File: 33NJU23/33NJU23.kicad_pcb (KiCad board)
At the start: 2 copper layers, 54 x 85.7 mm, 75 parts, among them CN1 HDMI, J1 VGA, J10 Conn_01x02, J11 Conn_01x01, J12 Audio OUT, J13 Audio IN, J14 JOY-1, J15 USB_A, J17 USB_B_Micro, J18 Conn_01x02_Female, J2 EXT, J3 Micro_SD_Card, J4 Conn_SD, J5 PWR, J6 UART, J7 Mini-DIN-6, J8 IN_A, J9 IN_A, Q1 BC850, Q2 BC850, U1 raspberrypi-pico-module

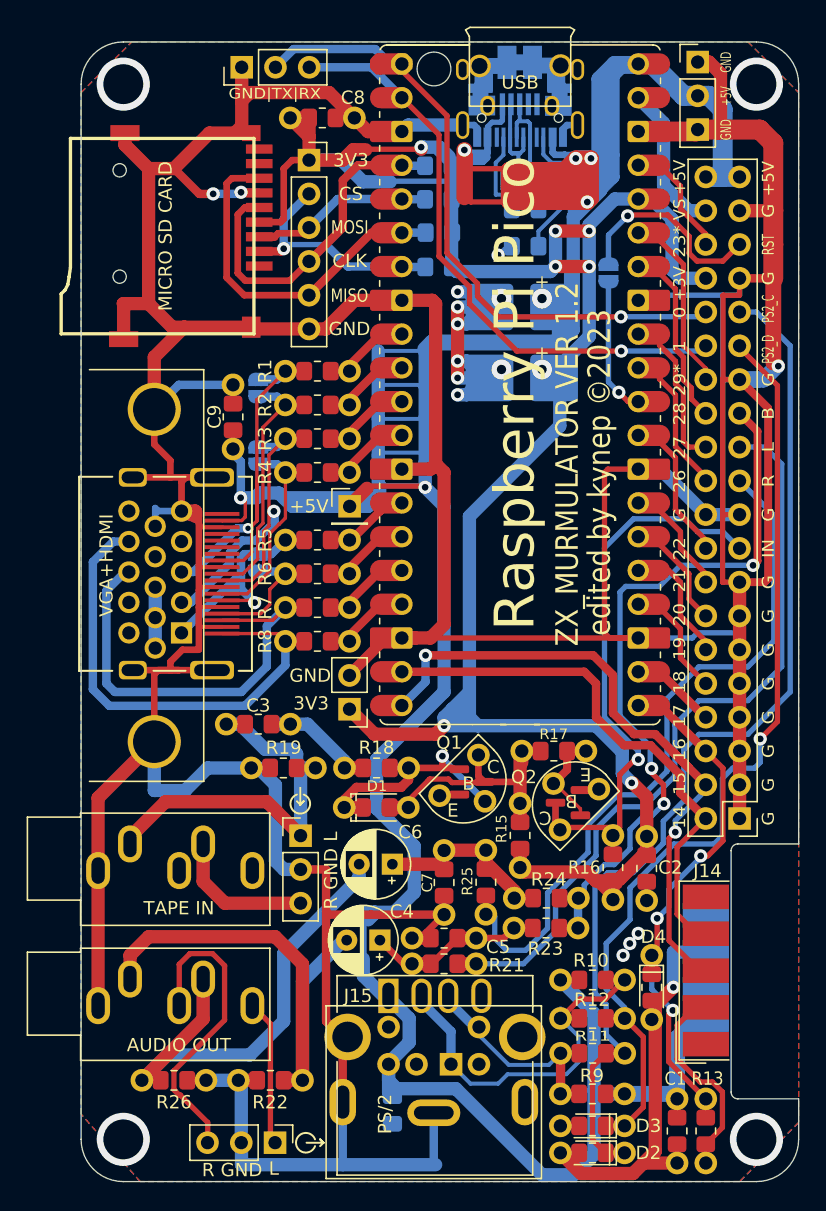
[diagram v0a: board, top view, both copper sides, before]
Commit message: logo
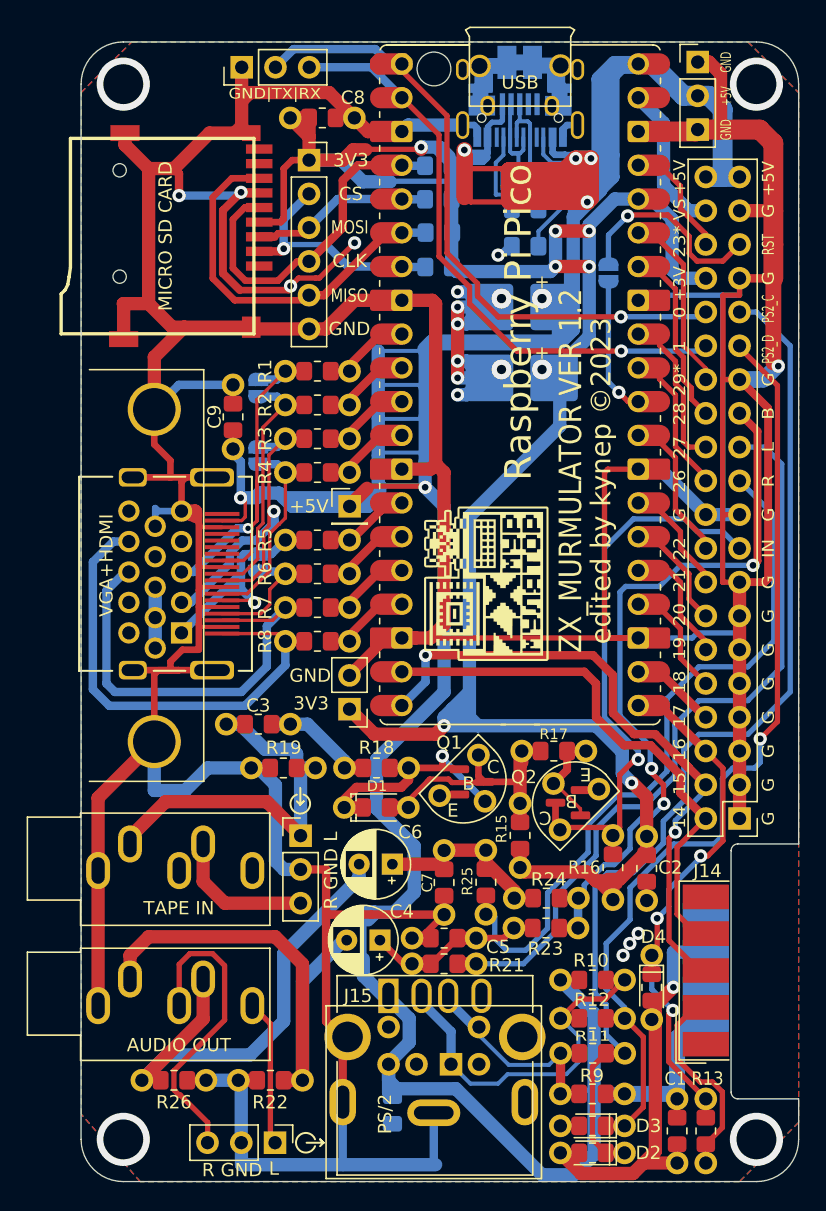
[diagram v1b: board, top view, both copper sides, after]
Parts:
- added G***: LOGO, LOGO, F.Cu at (60.3, 68.7)
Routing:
- net GND: track 554.6 -> 574.3 mm, vias 16 -> 18
- net /GP_4: track 27.8 -> 30.6 mm
